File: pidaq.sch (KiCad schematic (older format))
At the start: 7 parts, among them J5 Conn_01x03_Male, J6 Conn_01x08_Female, U3 SN74LV1T34DCKR

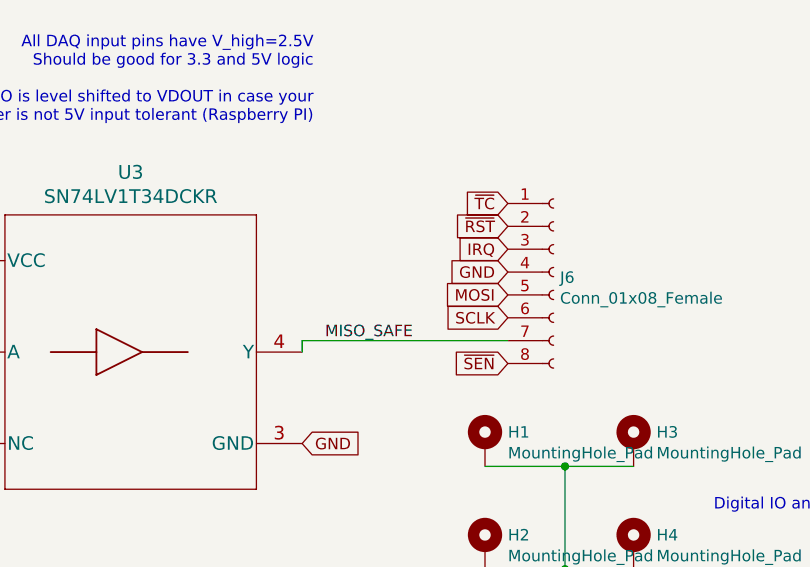
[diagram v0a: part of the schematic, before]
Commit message: completed design 2.0
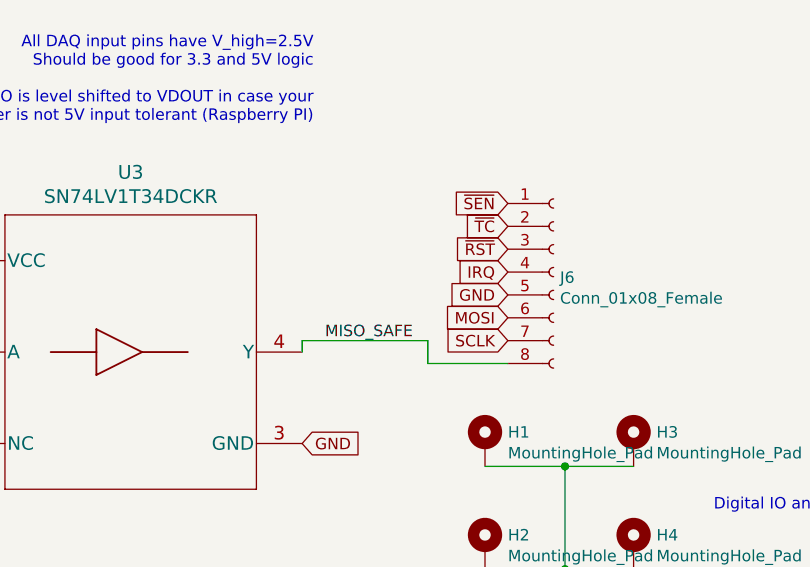
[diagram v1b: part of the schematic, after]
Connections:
- net GND: now also J6.5 (Pin_5); no longer J6.4 (Pin_4)
- net IRQ: now also J6.4 (Pin_4); no longer J6.3 (Pin_3)
- net MISO_SAFE: now also J6.8 (Pin_8); no longer J6.7 (Pin_7)
- net MOSI: now also J6.6 (Pin_6); no longer J6.5 (Pin_5)
- net SCLK: now also J6.7 (Pin_7); no longer J6.6 (Pin_6)
- net ~RST: now also J6.3 (Pin_3); no longer J6.2 (Pin_2)
- net ~SEN: now also J6.1 (Pin_1); no longer J6.8 (Pin_8)
- net ~TC: now also J6.2 (Pin_2); no longer J6.1 (Pin_1)
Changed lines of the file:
@@
 	1    0    0    -1
 $EndComp
-Text GLabel 9150 2900 0    50   Input ~ 0
+Text GLabel 9150 2200 0    50   Input ~ 0
 ~SEN
-Text GLabel 9150 2400 0    50   Input ~ 0
+Text GLabel 9150 2500 0    50   Input ~ 0
 IRQ
-Text GLabel 9150 2500 0    50   Input ~ 0
+Text GLabel 9150 2600 0    50   Input ~ 0
 GND
+Text GLabel 9150 2800 0    50   Input ~ 0
+SCLK
 Text GLabel 9150 2700 0    50   Input ~ 0
-SCLK
-Text GLabel 9150 2600 0    50   Input ~ 0
 MOSI
 Text GLabel 6750 2850 0    50   Input ~ 0
@@
 GND
 Wire Wire Line
-	9150 2800 8250 2800
-Wire Wire Line
 	8250 2800 8250 2850
 Wire Notes Line
@@
 Text Label 8350 2800 0    50   ~ 0
 MISO_SAFE
-Text GLabel 9150 2200 0    50   Input ~ 0
+Text GLabel 9150 2300 0    50   Input ~ 0
 ~TC
 $Comp
@@
 Text GLabel 4600 4850 2    50   Input ~ 0
 ~RST
-Text GLabel 9150 2300 0    50   Input ~ 0
+Text GLabel 9150 2400 0    50   Input ~ 0
 ~RST
+Wire Wire Line
+	8250 2800 8800 2800
+Wire Wire Line
+	8800 2800 8800 2900
+Wire Wire Line
+	8800 2900 9150 2900
 $EndSCHEMATC
